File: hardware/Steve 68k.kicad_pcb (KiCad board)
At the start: 2 copper layers, 99 x 98.9 mm, 56 parts, among them IC1 MC68008FN8, J1 Conn_02x32_Odd_Even, J2 5V Input, J3 Serial 1, J4 CLK Select, J6 Serial 2, SW1 Reset, U1 74LS32, U2 28C256, U3 GAL16V8, U4 74HC04, U5 MC68681FN, U6 L7805, U7 AS6C4008-55PCN, U8 Max705, X1 CXO_DIP8, Y1 3.6864

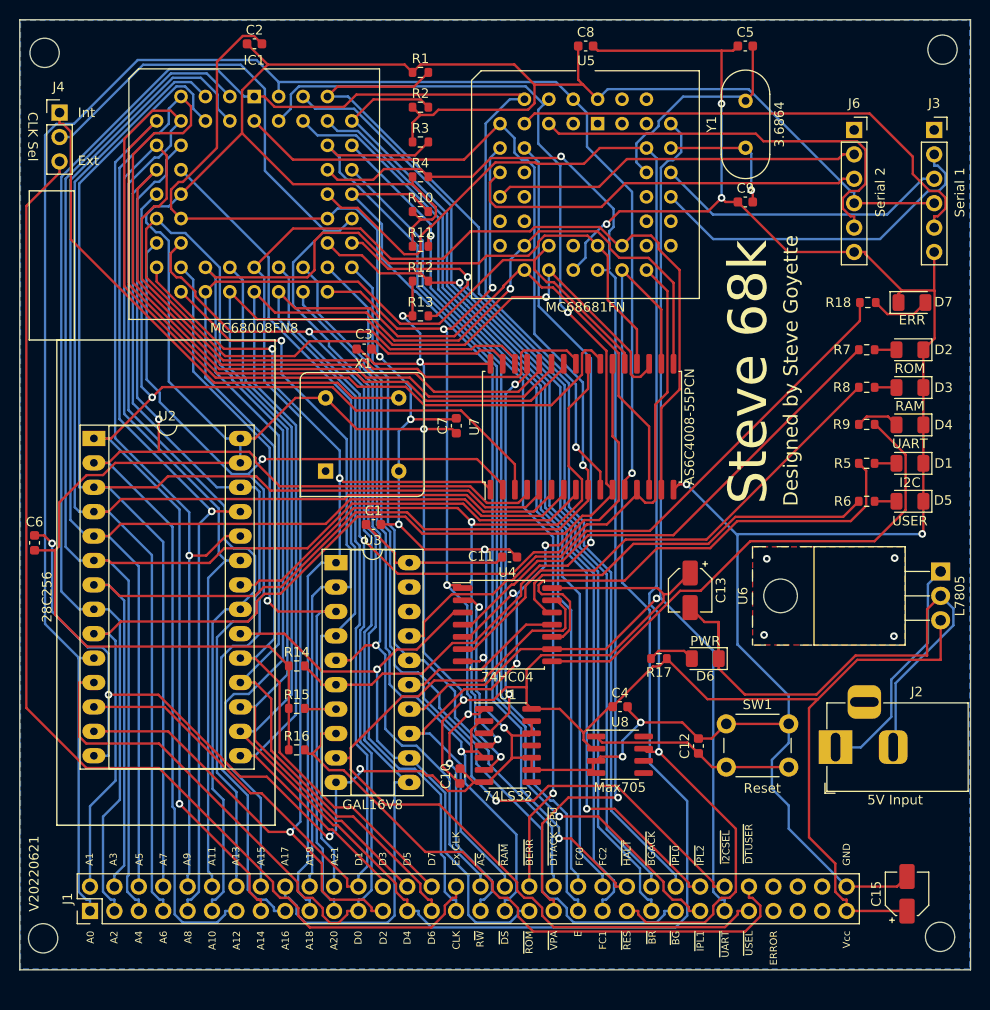
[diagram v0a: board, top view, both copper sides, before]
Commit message: V20220905 sent for fab
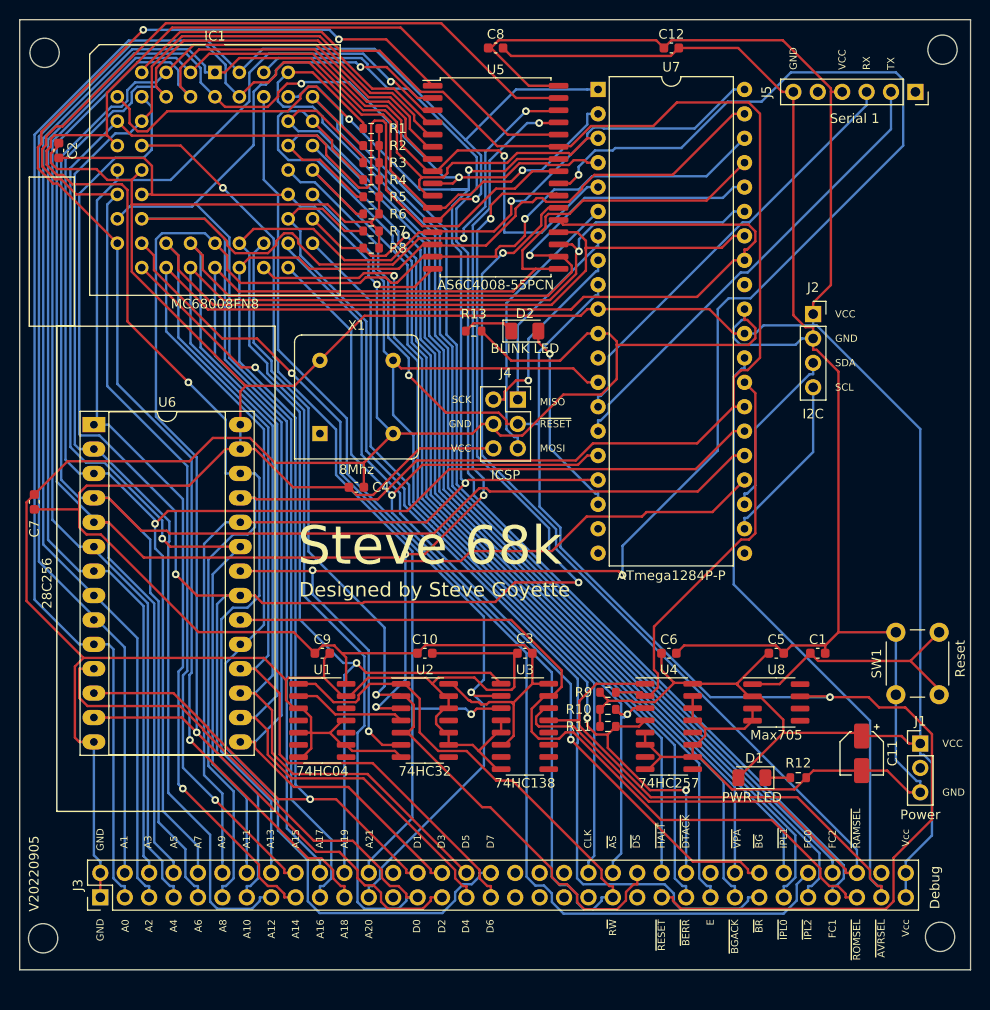
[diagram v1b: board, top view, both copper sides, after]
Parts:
- removed C13: 100uF, Capacitor_SMD:CP_Elec_4x5.4
- removed C15: 10uF, Capacitor_SMD:CP_Elec_4x5.4
- removed D3: RAM, LED_SMD:LED_1206_3216Metric
- removed D4: UART, LED_SMD:LED_1206_3216Metric
- removed D5: USER, LED_SMD:LED_1206_3216Metric
- removed D6: PWR, LED_SMD:LED_1206_3216Metric
- removed D7: ERR, LED_SMD:LED_1206_3216Metric
- removed J6: Serial 2, Connector_PinSocket_2.54mm:PinSocket_1x06_P2.54mm_Vertical
- removed R14, R15, R16: 10k, Resistor_SMD:R_0603_1608Metric
- removed R17, R18: 220, Resistor_SMD:R_0603_1608Metric
- removed the U6 at (159.6, 93.9)
- removed Y1: 3.6864, Crystal:Crystal_HC49-U_Vertical
- added J5: Serial 1, Connector_PinSocket_2.54mm:PinSocket_1x06_P2.54mm_Vertical, F.Cu at (157.0, 43.9)
- added U2: 74HC32, Package_SO:SOIC-14_3.9x8.7mm_P1.27mm, F.Cu at (105.9, 109.4)
- C1: value .1uF -> 100nf
- C11: value .1uF -> 100uF; footprint Capacitor_SMD:C_0603_1608Metric -> Capacitor_SMD:CP_Elec_4x5.4
- C12: value 100nf -> .1uF
- C5, C9: value 12pf -> .1uF
- D1: value I2C -> PWR LED
- D2: value ROM -> BLINK LED
- J1: value Conn_02x32_Odd_Even -> Power; footprint Connector_PinHeader_2.54mm:PinHeader_2x32_P2.54mm_Vertical -> Connector_PinHeader_2.54mm:PinHeader_1x03_P2.54mm_Vertical
- J2: value 5V Input -> I2C; footprint Connector_BarrelJack:BarrelJack_Horizontal -> Connector_PinSocket_2.54mm:PinSocket_1x04_P2.54mm_Vertical
- J3: value Serial 1 -> Debug; footprint Connector_PinSocket_2.54mm:PinSocket_1x06_P2.54mm_Vertical -> Connector_PinHeader_2.54mm:PinHeader_2x34_P2.54mm_Vertical
- J4: value CLK Select -> ICSP; footprint Connector_PinHeader_2.54mm:PinHeader_1x03_P2.54mm_Vertical -> Connector_PinSocket_2.54mm:PinSocket_2x03_P2.54mm_Vertical
- R12, R13: value 10k -> 220
- R5, R6, R7, R8, R9: value 220 -> 10k
- U1: value 74LS32 -> 74HC04
- U3: value GAL16V8 -> 74HC138; footprint Package_DIP:DIP-20_W7.62mm_Socket_LongPads -> Package_SO:SOIC-16_3.9x9.9mm_P1.27mm
- U4: value 74HC04 -> 74HC257; footprint Package_SO:SOIC-14W_7.5x9mm_P1.27mm -> Package_SO:SOIC-16_3.9x9.9mm_P1.27mm
- U5: value MC68681FN -> AS6C4008-55PCN; footprint Package_LCC:PLCC-44_THT-Socket -> Package_SO:SSOP-32_11.305x20.495mm_P1.27mm
- U7: value AS6C4008-55PCN -> ATmega1284P-P; footprint Package_SO:SSOP-32_11.305x20.495mm_P1.27mm -> Package_DIP:DIP-40_W15.24mm
- X1: value CXO_DIP8 -> 8Mhz
- moved J3 117.9 mm to (72.1, 127.8), turned to 90 degrees
- moved J1 88.2 mm to (157.5, 111.8), turned to 0 degrees
- moved C12 72.7 mm to (131.6, 39.4), turned to 0 degrees
- moved C6 67.0 mm to (131.3, 102.4), turned to 0 degrees
- moved R12 64.9 mm to (144.8, 115.3), turned to 180 degrees
- moved C9 64.4 mm to (95.2, 102.4)
- moved C5 63.3 mm to (142.5, 102.4)
- moved R6 59.6 mm to (100.3, 56.6), turned to 180 degrees
- moved R5 58.6 mm to (100.3, 54.9), turned to 180 degrees
- moved J4 56.3 mm to (115.6, 76.0)
- moved R10 55.4 mm to (125.0, 108.2)
- moved R11 53.6 mm to (125.0, 110.0)
- moved R8 53.6 mm to (100.3, 60.2), turned to 180 degrees
- moved R7 53.0 mm to (100.3, 58.4), turned to 180 degrees
- moved C1 48.1 mm to (146.8, 102.4)
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- renumbered U2 to U6
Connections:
- C1 pad 1: VCC -> Net-(C1-Pad1)
- C12 pad 1: Net-(C12-Pad1) -> VCC
- C5 pad 1: GND -> VCC
- C5 pad 2: /68681_X1 -> GND
- C9 pad 1: GND -> VCC
- C9 pad 2: /68681_X2 -> GND
- D1 pad 1: GND -> Net-(D1-Pad1)
- D1 pad 2: Net-(D1-Pad2) -> VCC
- D2 pad 1: GND -> Net-(D2-Pad1)
- IC1 pad 43: /68681_Int -> /~{VPA}
- J1 pad 1: /A0 -> VCC
- J1 pad 2: /A1 -> unconnected-(J1-Pad2)
- J1 pad 3: /A2 -> GND
- J2 pad 1: Net-(J2-Pad1) -> VCC
- J2 pad 2: Net-(C13-Pad2) -> GND
- J2 pad 3: (no net) -> /SDA
- J3 pad 1: /DTRA -> GND
- J3 pad 2: /TxDA -> GND
- J3 pad 3: /RxDA -> /A0
- J3 pad 4: VCC -> /A1
- J3 pad 5: /CTSA -> /A2
- J3 pad 6: GND -> /A3
- J4 pad 1: /CLK_ONBOARD -> /MISO
- J4 pad 2: /CLK -> /SCK
- J4 pad 3: /CLK_EXTERNAL -> /~{RESET}
- R10 pad 2: /~{HALT} -> /~{AS}
- R11 pad 2: /~{BERR} -> /~{DTACK_CPU}
- R12 pad 1: VCC -> GND
- R12 pad 2: /~{BR} -> Net-(D1-Pad1)
- R13 pad 1: VCC -> GND
- R13 pad 2: /~{BGACK} -> Net-(D2-Pad1)
- R4 pad 2: /68681_Int -> /~{BERR}
- R5 pad 1: Net-(R5-Pad1) -> VCC
- R5 pad 2: Net-(D1-Pad2) -> /~{VPA}
- R6 pad 1: Net-(R6-Pad1) -> VCC
- R6 pad 2: Net-(D5-Pad2) -> /~{HALT}
- R7 pad 1: Net-(R7-Pad1) -> VCC
- R7 pad 2: Net-(D2-Pad2) -> /~{BR}
- R8 pad 1: Net-(R8-Pad1) -> VCC
- R8 pad 2: Net-(D3-Pad2) -> /~{BGACK}
- R9 pad 1: Net-(R9-Pad1) -> VCC
- R9 pad 2: Net-(D4-Pad2) -> /~{DTACK_AVR}
- SW1 pad 2: Net-(C12-Pad1) -> Net-(C1-Pad1)
- U1 pad 10: GND -> unconnected-(U1-Pad10)
- U1 pad 11: unconnected-(U1-Pad11) -> GND
- U1 pad 12: GND -> unconnected-(U1-Pad12)
- U1 pad 2: /~{DS} -> Net-(U1-Pad2)
- U1 pad 3: /~{RAM_WE} -> GND
- U1 pad 4: Net-(U1-Pad4) -> unconnected-(U1-Pad4)
- U1 pad 5: /~{DS} -> GND
- U1 pad 6: /~{OE} -> unconnected-(U1-Pad6)
- U3 pad 1: /A18 -> /A19
- U3 pad 10: GND -> unconnected-(U3-Pad10)
- U3 pad 11: /A17 -> unconnected-(U3-Pad11)
- U3 pad 12: /~{ROMSEL} -> unconnected-(U3-Pad12)
- U3 pad 13: /~{RAMSEL} -> /~{AVRSEL}
- U3 pad 14: /~{UARTSEL} -> /~{RAMSEL}
- U3 pad 15: /~{I2CSEL} -> /~{ROMSEL}
- U3 pad 16: /~{DTACK_CPU} -> VCC
- U3 pad 2: /A19 -> /A20
- U3 pad 3: /A20 -> /A21
- U3 pad 4: /A21 -> GND
- U3 pad 5: /~{AS} -> GND
- U3 pad 6: /~{DTACK_UART} -> VCC
- U3 pad 7: /~{DTACK_I2C} -> unconnected-(U3-Pad7)
- U3 pad 8: /~{DTACK_USER} -> GND
- U3 pad 9: /~{USERSEL} -> unconnected-(U3-Pad9)
- U4 pad 1: /R~{W} -> /~{AVRSEL}
- U4 pad 10: Net-(R5-Pad1) -> GND
- U4 pad 11: /~{I2CSEL} -> GND
- U4 pad 12: Net-(R6-Pad1) -> unconnected-(U4-Pad12)
- U4 pad 13: /~{USERSEL} -> GND
- U4 pad 14: VCC -> GND
- U4 pad 2: Net-(U1-Pad4) -> /~{DTACK_AVR}
- U4 pad 3: /~{ROMSEL} -> /~{AS}
- U4 pad 4: Net-(R7-Pad1) -> /~{DTACK_CPU}
- U4 pad 5: /~{RAMSEL} -> GND
- U4 pad 6: Net-(R8-Pad1) -> GND
- U4 pad 7: GND -> unconnected-(U4-Pad7)
- U4 pad 8: Net-(R9-Pad1) -> GND
- U4 pad 9: /~{UARTSEL} -> unconnected-(U4-Pad9)
- U5 pad 1: unconnected-(U5-Pad1) -> /A18
- U5 pad 10: /~{DTACK_UART} -> /A2
- U5 pad 11: /RxDB -> /A1
- U5 pad 12: unconnected-(U5-Pad12) -> /A0
- U5 pad 13: /TxDB -> /D0
- U5 pad 14: /OP1 -> /D1
- U5 pad 15: /OP3 -> /D2
- U5 pad 16: /OP5 -> GND
- U5 pad 17: /OP7 -> /D3
- U5 pad 18: /D1 -> /D4
- U5 pad 19: /D3 -> /D5
- U5 pad 2: /A0 -> /A16
- U5 pad 20: /D5 -> /D6
- U5 pad 22: GND -> /~{RAMSEL}
- U5 pad 23: unconnected-(U5-Pad23) -> /A10
- U5 pad 24: /68681_Int -> /~{OE}
- U5 pad 25: /D6 -> /A11
- U5 pad 26: /D4 -> /A9
- U5 pad 27: /D2 -> /A8
- U5 pad 28: /D0 -> /A13
- U5 pad 29: /OP6 -> /~{RAM_WE}
- U5 pad 3: /IP3 -> /A14
- U5 pad 30: /OP4 -> /A17
- U5 pad 31: /RTSB -> /A15
- U5 pad 32: /RTSA -> VCC
- U5 pad 4: /A1 -> /A12
- U5 pad 5: /CTSB -> /A7
- U5 pad 6: /A2 -> /A6
- U5 pad 7: /A3 -> /A5
- U5 pad 8: /CTSA -> /A4
- U5 pad 9: /R~{W} -> /A3
- U7 pad 1: /A18 -> /A0
- U7 pad 10: /A2 -> VCC
- U7 pad 11: /A1 -> GND
- U7 pad 12: /A0 -> unconnected-(U7-Pad12)
- U7 pad 13: /D0 -> /CLK
- U7 pad 14: /D1 -> /RXD0
- U7 pad 15: /D2 -> /TXD0
- U7 pad 16: GND -> /R~{W}
- U7 pad 17: /D3 -> /A9
- U7 pad 18: /D4 -> Net-(D2-Pad2)
- U7 pad 19: /D5 -> /IPL0
- U7 pad 2: /A16 -> /A1
- U7 pad 20: /D6 -> /IPL1
- U7 pad 21: /D7 -> /IPL2
- U7 pad 22: /~{RAMSEL} -> /SCL
- U7 pad 23: /A10 -> /SDA
- U7 pad 24: /~{OE} -> /A5
- U7 pad 25: /A11 -> /A6
- U7 pad 26: /A9 -> /A7
- U7 pad 28: /A13 -> /~{DTACK_AVR}
- U7 pad 29: /~{RAM_WE} -> /~{AVRSEL}
- U7 pad 3: /A14 -> /A2
- U7 pad 30: /A17 -> VCC
- U7 pad 31: /A15 -> GND
- U7 pad 32: VCC -> unconnected-(U7-Pad32)
- U7 pad 4: /A12 -> /A3
- U7 pad 5: /A7 -> /A4
- U7 pad 6: /A6 -> /MOSI
- U7 pad 7: /A5 -> /MISO
- U7 pad 8: /A4 -> /SCK
- U7 pad 9: /A3 -> /~{RESET}
- U8 pad 1: Net-(C12-Pad1) -> Net-(C1-Pad1)
- X1 pad 5: /CLK_ONBOARD -> /CLK
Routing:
- net /~{UARTSEL}: track 117.5 -> 0.00 mm, vias 1 -> 0
- net /~{AVRSEL}: track 0.00 -> 116.7 mm
- net /CLK_EXTERNAL: track 116.5 -> 0.00 mm
- net /68681_Int: track 116.0 -> 0.00 mm, vias 2 -> 0
- net /~{VPA}: track 0.00 -> 108.2 mm
- net GND: track 440.8 -> 528.6 mm, vias 21 -> 1
- net /~{OE}: track 84.3 -> 169.5 mm, vias 2 -> 4
- net /~{USERSEL}: track 85.2 -> 0.00 mm
- net /~{DTACK_UART}: track 81.5 -> 0.00 mm, vias 1 -> 0
- net /~{DTACK_USER}: track 64.7 -> 0.00 mm
- net /ERROR: track 63.2 -> 0.00 mm
- net /~{I2CSEL}: track 63.2 -> 0.00 mm, vias 1 -> 0
- net Net-(C13-Pad2): track 62.3 -> 0.00 mm
- net /A5: track 154.2 -> 211.0 mm
- net /A6: track 150.5 -> 207.1 mm
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- removed copper zone on B.Cu, net GND
- removed copper zone on F.Cu, net GND
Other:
- board text added: "MISO"
- board text added: "MOSI"
- board text added: "RX"
- board text added: "SCK"
- board text added: "SCL"
- board text added: "SDA"
- board text added: "TX"
- board text added: "V20220905"
- board text added: "VCC"
- board text added: "~{AVRSEL}"
- board text added: "~{DTACK}"
- board text added: "~{RAMSEL}"
- board text added: "~{RESET}"
- board text added: "~{ROMSEL}"
- board text removed: "CLK Sel"
- board text removed: "ERROR"
- board text removed: "Ex CLK"
- board text removed: "Ext"
- board text removed: "Int"
- board text removed: "V20220621"
- board text removed: "~{DTACK_CPU}"
- board text removed: "~{DTUSER}"
- board text removed: "~{I2CSEL}"
- board text removed: "~{RAM}"
- board text removed: "~{RES}"
- board text removed: "~{ROM}"
- board text removed: "~{UART}"
- board text removed: "~{USEL}"
